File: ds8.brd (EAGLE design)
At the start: 85 x 50 mm, 87 parts, among them IC1 TM4C1230C3PM, IC2 TPS77333, Q1 BC850, Q2 BC850, Q3 BC850, U1 LM13700M, U2 LM324, U3 LM324, U4 LM741D

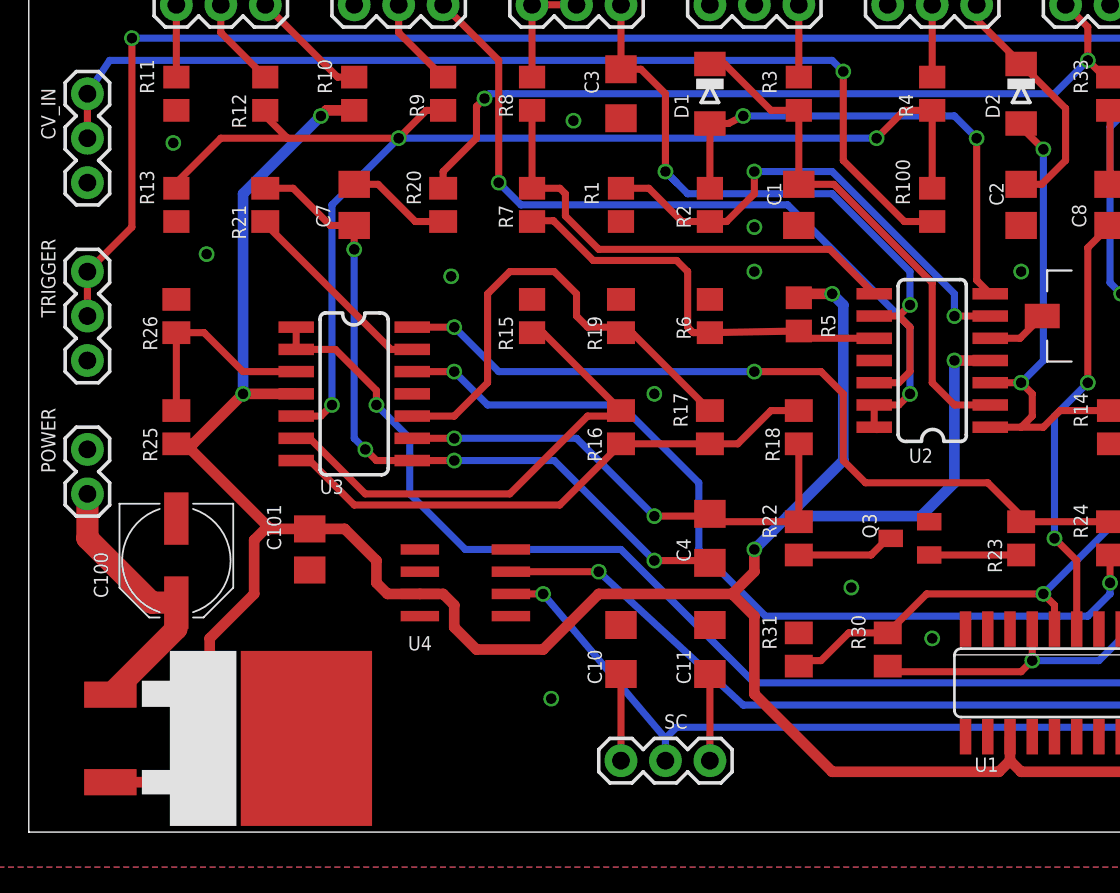
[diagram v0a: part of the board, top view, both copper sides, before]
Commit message: clean up
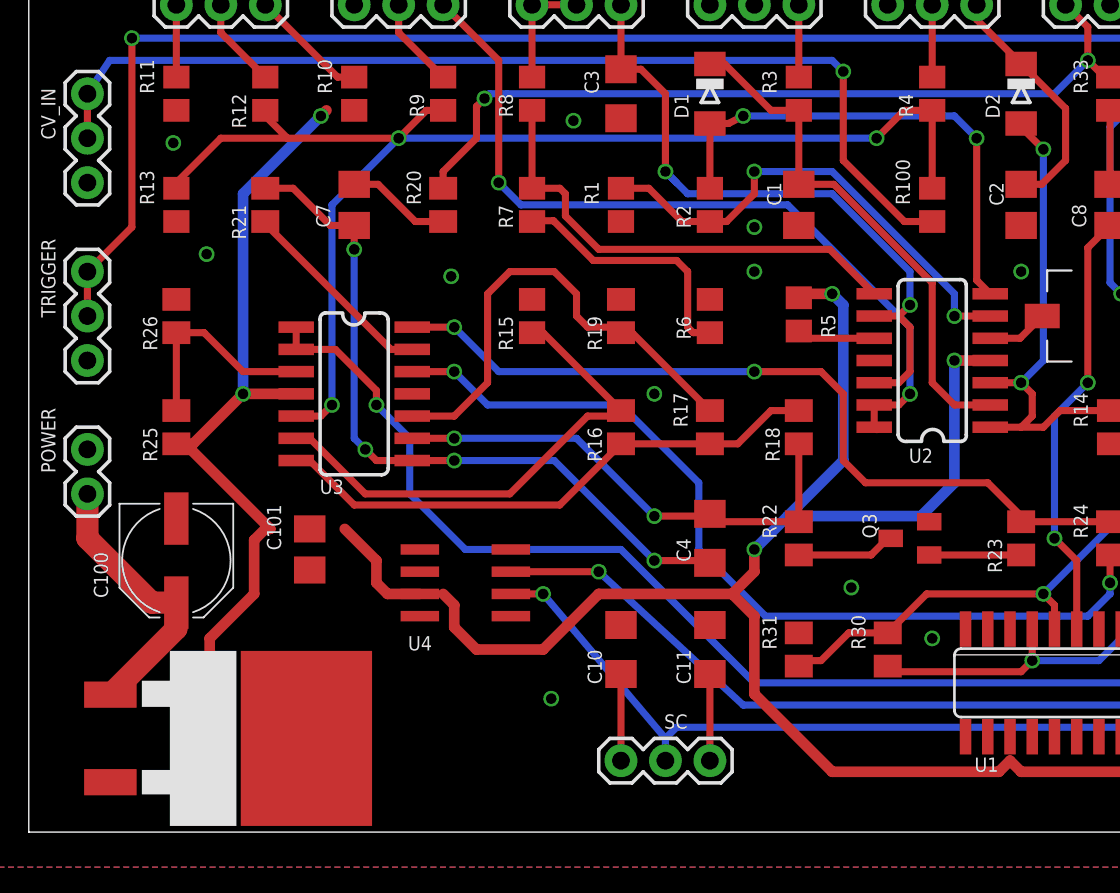
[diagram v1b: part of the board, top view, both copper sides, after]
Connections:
- removed net GNDA: IC1.3
- removed net N$18: IC1.42
- removed net N$35: IC1.54
- removed net VDDA: IC1.2
- net GND: now also IC1.3
- net N$5: no longer R5.2
- net VCC: now also R5.2; no longer R5.1
- net VDD: now also IC1.2, IC1.42, IC1.54
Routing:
- net VCC: track 181.4 -> 166.9 mm
- net N$5: track 24.5 -> 18.9 mm
